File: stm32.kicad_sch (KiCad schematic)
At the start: 31 parts, among them J201 Conn_ST_STDC14, J203 GPIO, J204 I2C2, J205 UART1, U201 STM32G431KBT6, U202 ADXL343, Y201 16MHz

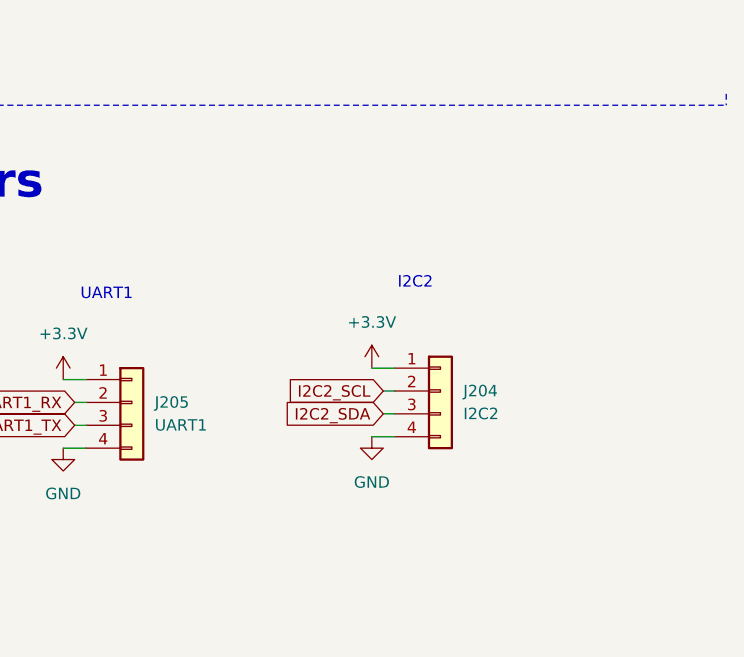
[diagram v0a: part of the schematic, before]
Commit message: First rev by M. FIACK
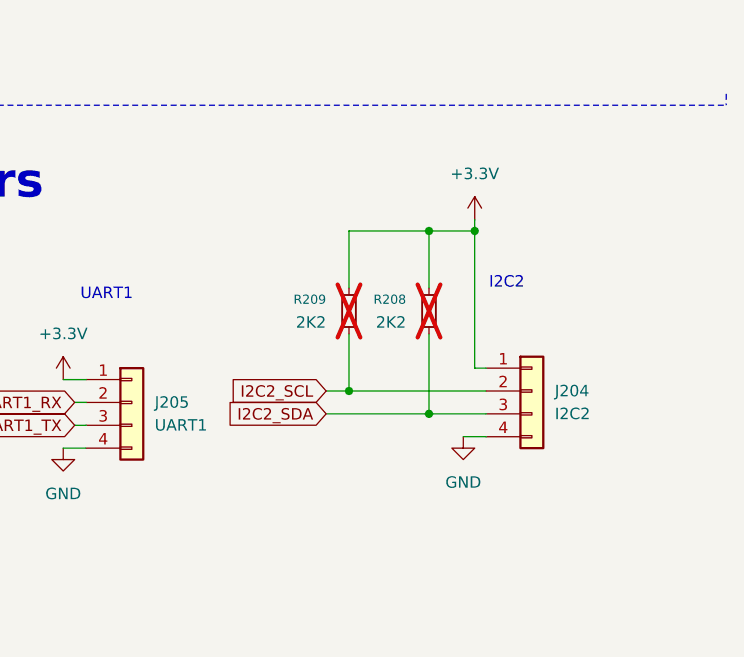
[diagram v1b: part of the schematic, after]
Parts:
- added R208, R209: 2K2, Resistor_SMD:R_0603_1608Metric, symbol Device:R_Small
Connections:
- net +3.3V: now also R208.1, R209.1
- net I2C2_SCL: now also R209.2
- net I2C2_SDA: now also R208.2
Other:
- moved on the sheet: J204
